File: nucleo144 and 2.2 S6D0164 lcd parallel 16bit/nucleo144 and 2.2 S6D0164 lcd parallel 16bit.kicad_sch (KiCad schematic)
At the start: 2 parts, among them U1 NUCLEO144

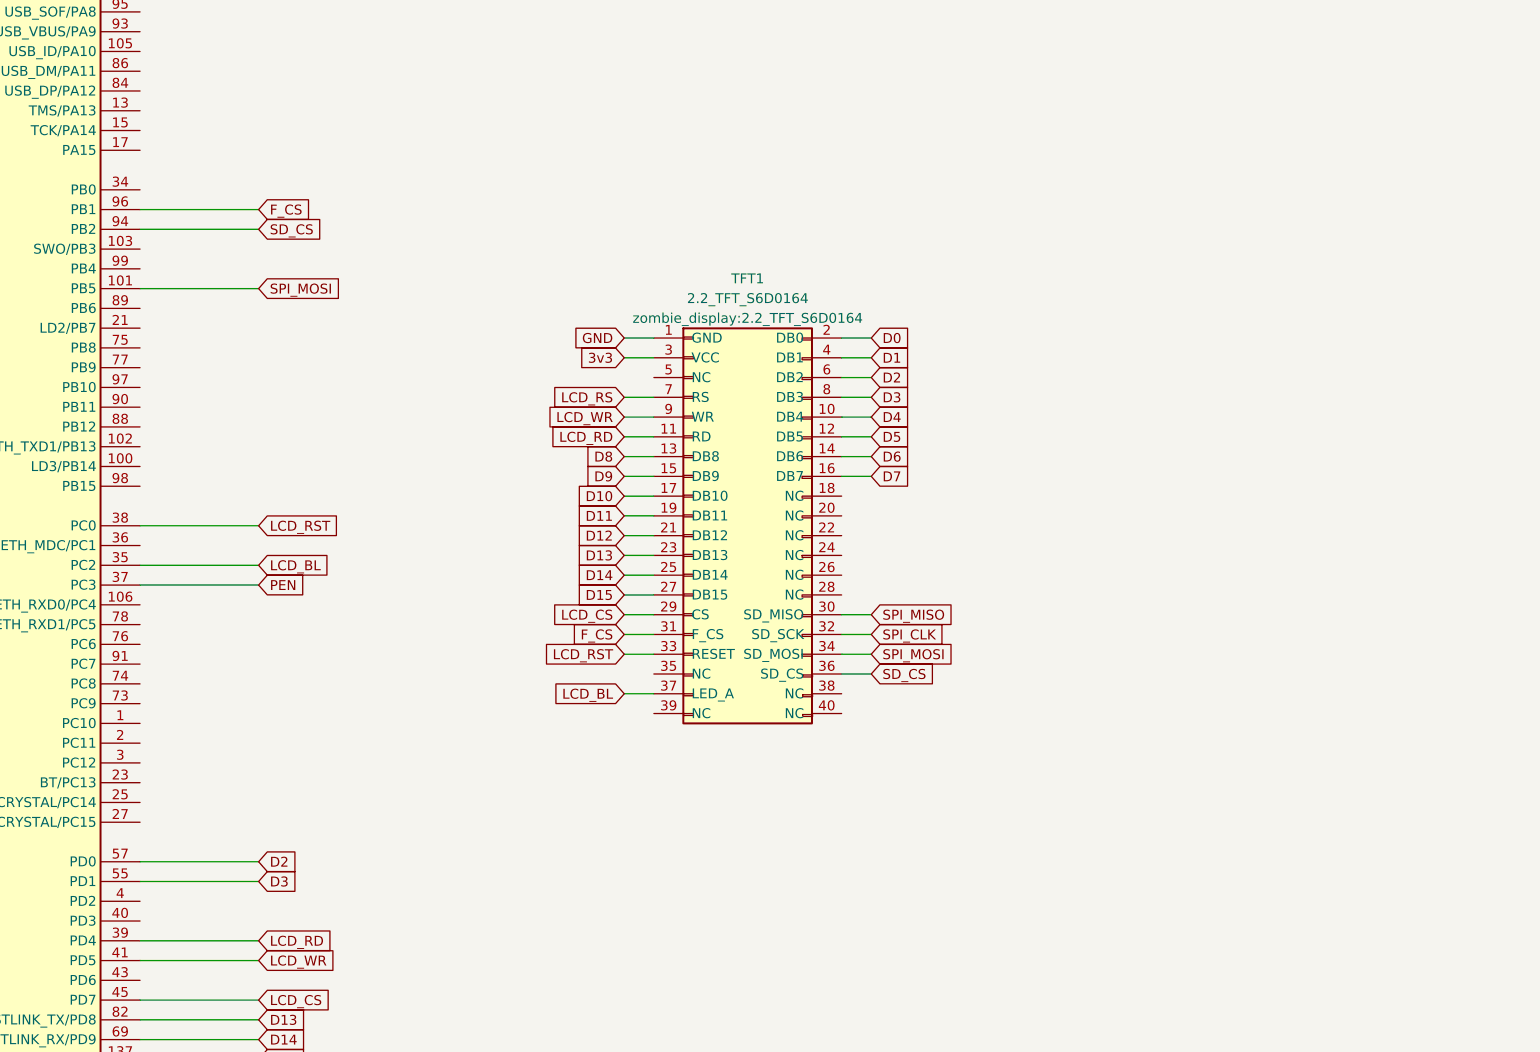
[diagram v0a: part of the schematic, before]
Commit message: Signed-off-by: DamianPodrazaCode <damian.podraza@gmail.com>
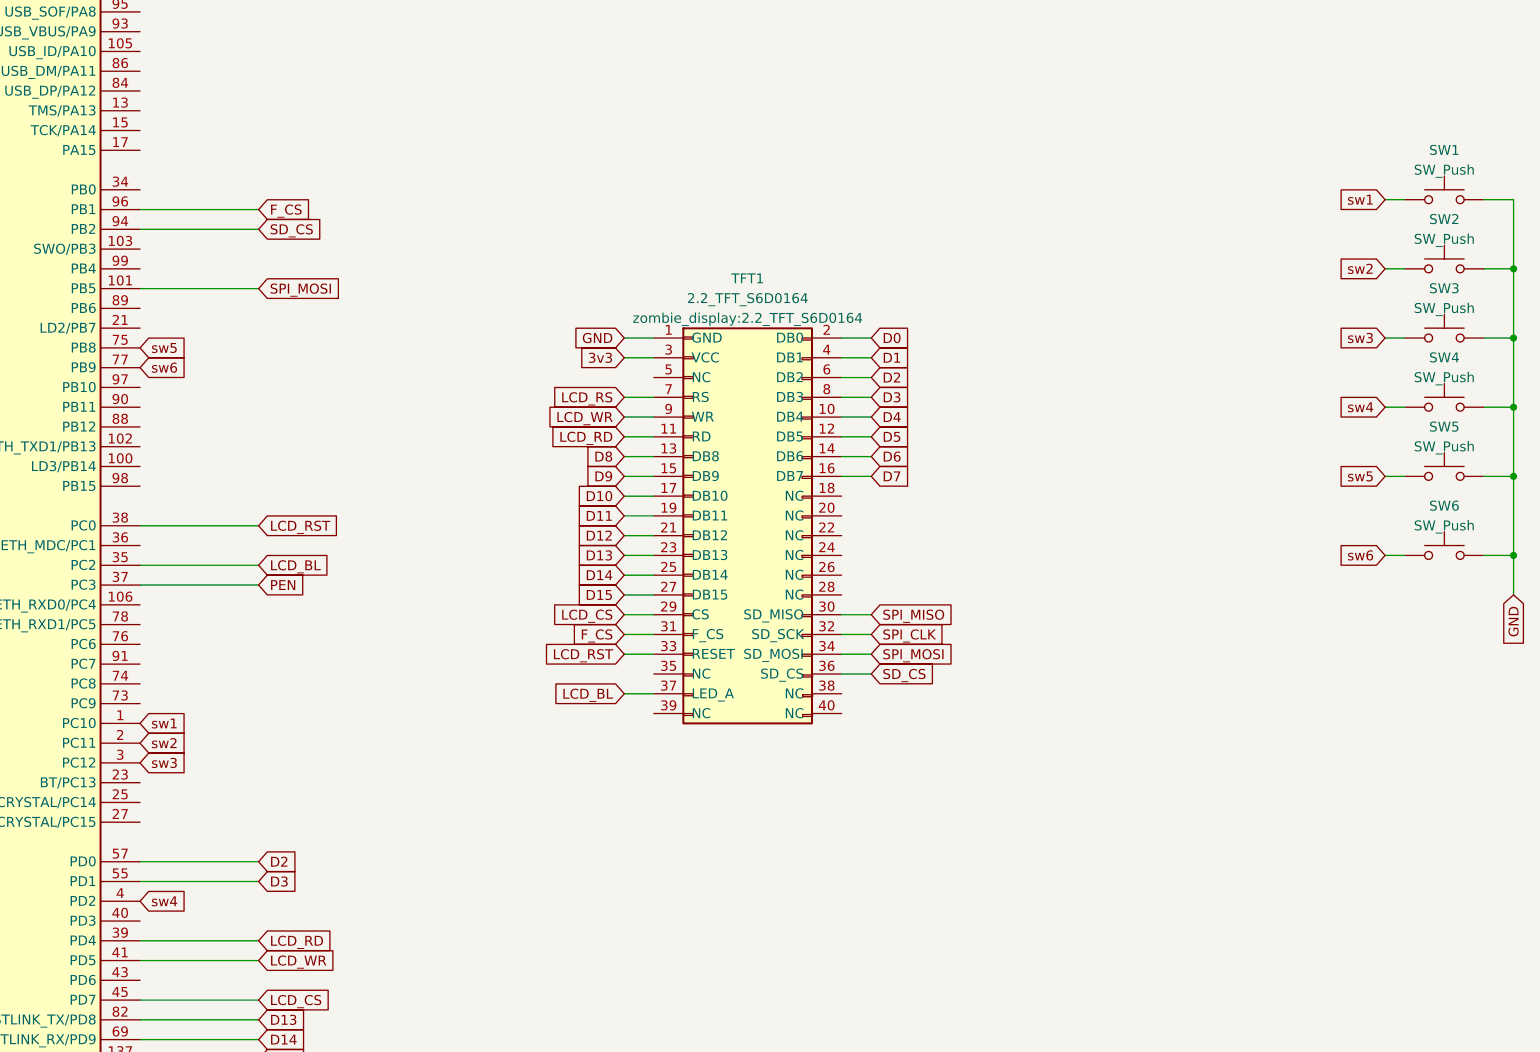
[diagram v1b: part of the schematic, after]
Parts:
- added SW1, SW2, SW3, SW4, SW5, SW6: SW_Push, Button_Switch_THT:SW_PUSH_6mm, symbol Switch:SW_Push
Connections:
- net GND: now also SW1.2, SW2.2, SW3.2, SW4.2, SW5.2, SW6.2
- net sw1: now reaches U1.1 (PC10)
- net sw1: now also SW1.1
- net sw2: now reaches U1.2 (PC11)
- net sw2: now also SW2.1
- net sw3: now reaches U1.3 (PC12)
- net sw3: now also SW3.1
- net sw4: now reaches U1.4 (PD2)
- net sw4: now also SW4.1
- net sw5: now reaches U1.75 (PB8)
- net sw5: now also SW5.1
- net sw6: now reaches U1.77 (PB9)
- net sw6: now also SW6.1

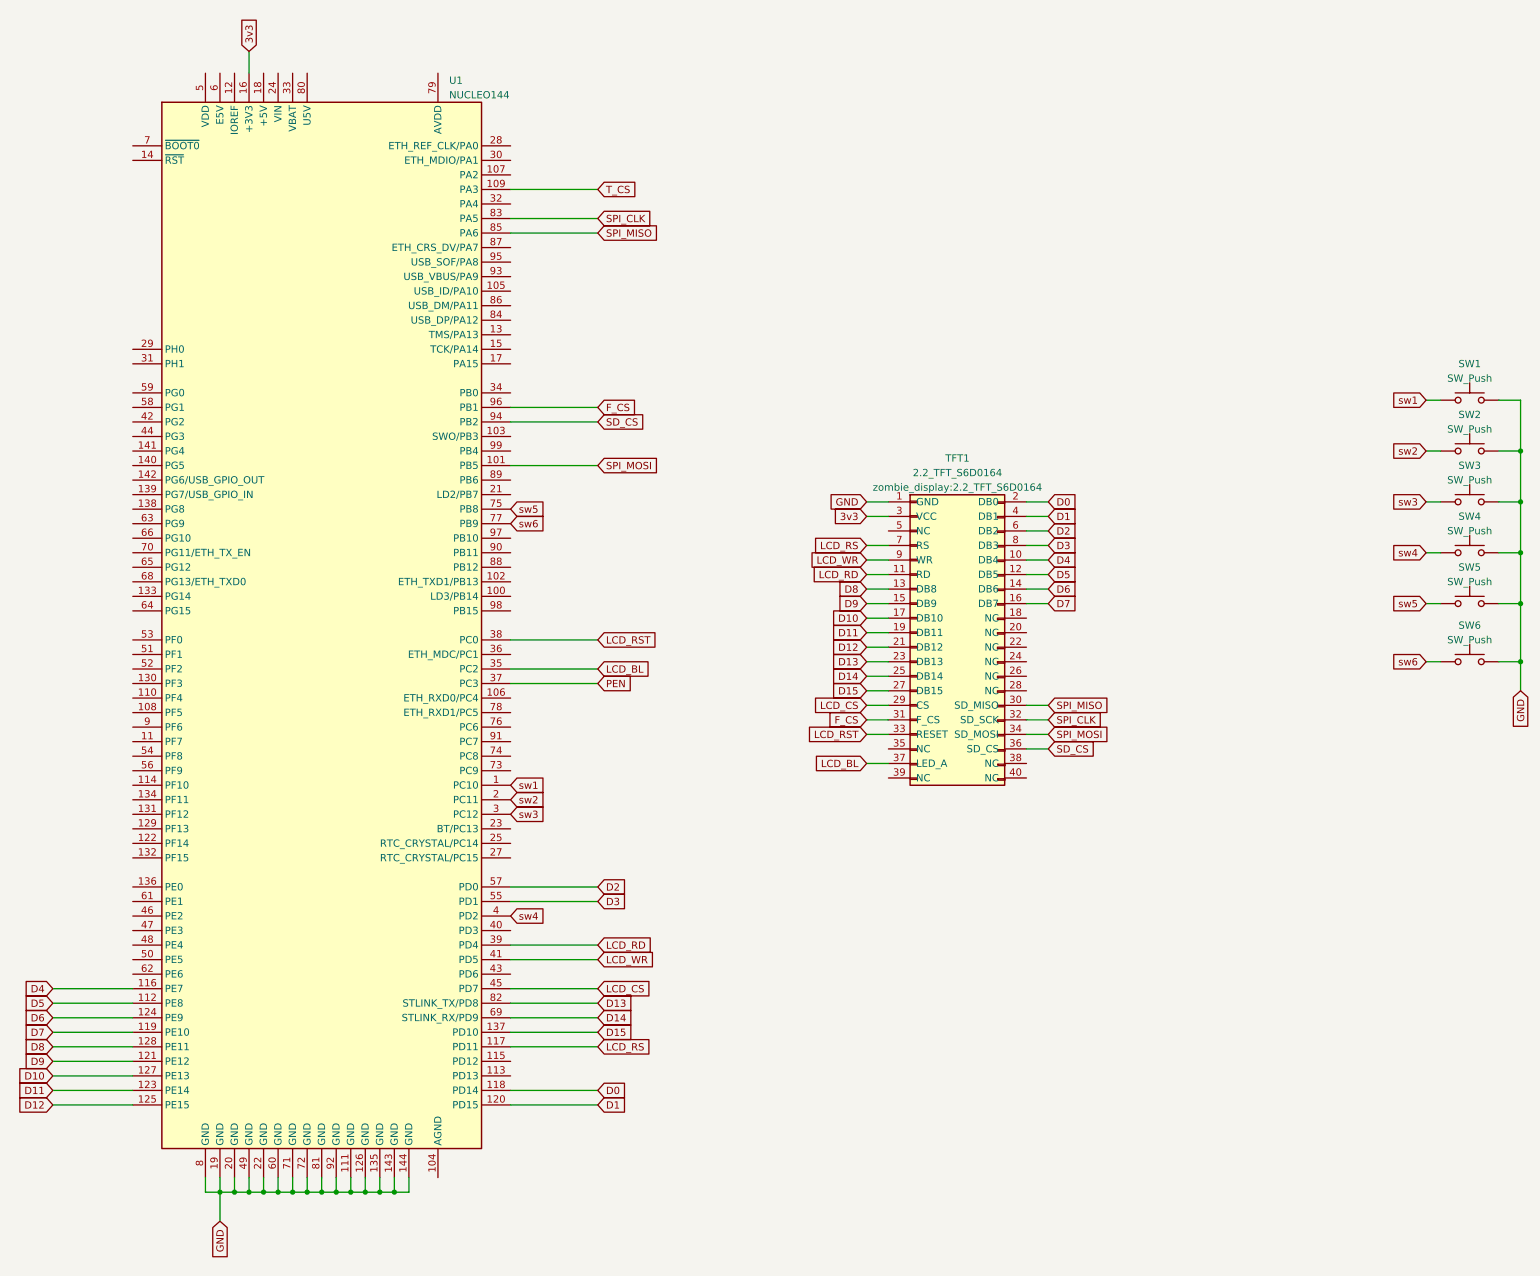
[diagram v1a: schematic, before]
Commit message: Signed-off-by: DamianPodrazaCode <damian.podraza@gmail.com>
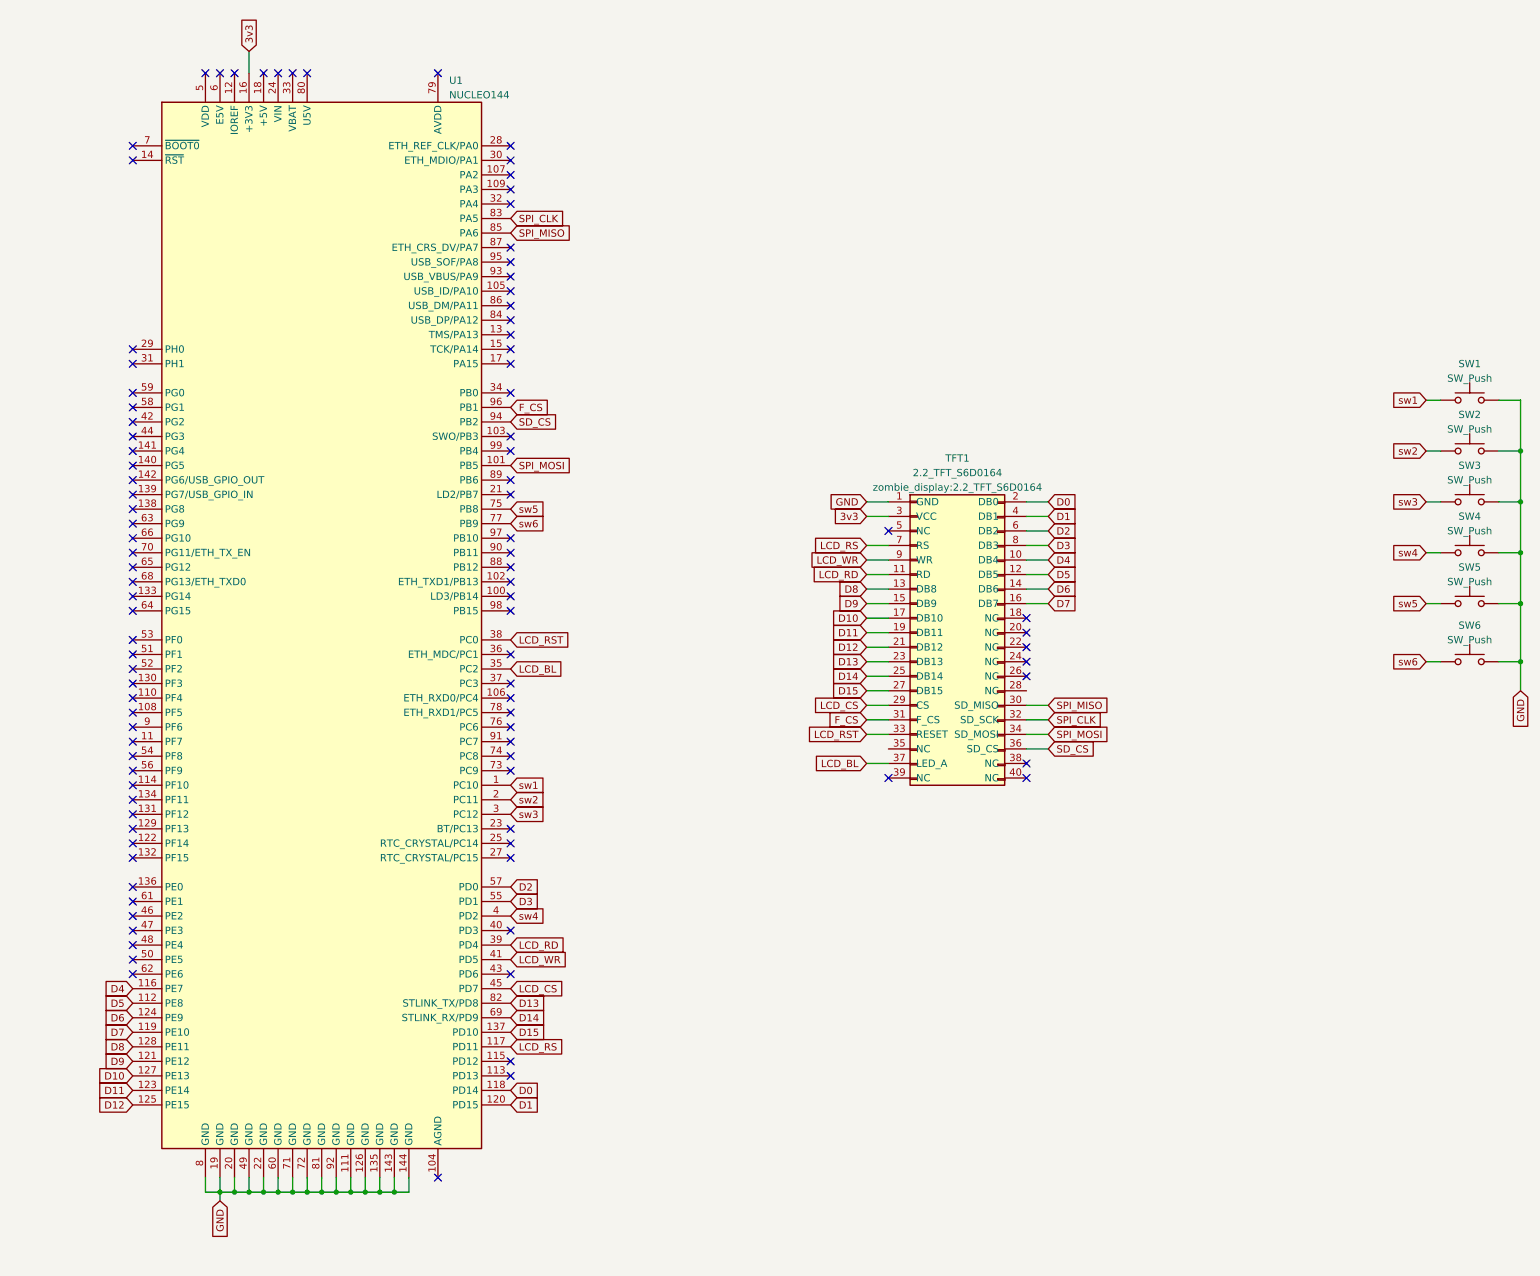
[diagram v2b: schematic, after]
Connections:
- net PEN: no longer names the net of U1.37 (PC3)
- net T_CS: no longer names the net of U1.109 (PA3)
- no-connect marks 0 -> 101
